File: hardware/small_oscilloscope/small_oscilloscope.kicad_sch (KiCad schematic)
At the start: 5 parts, among them J1 Conn_01x16, J2 Conn_01x16, J7 Conn_01x03, U1 CH423S

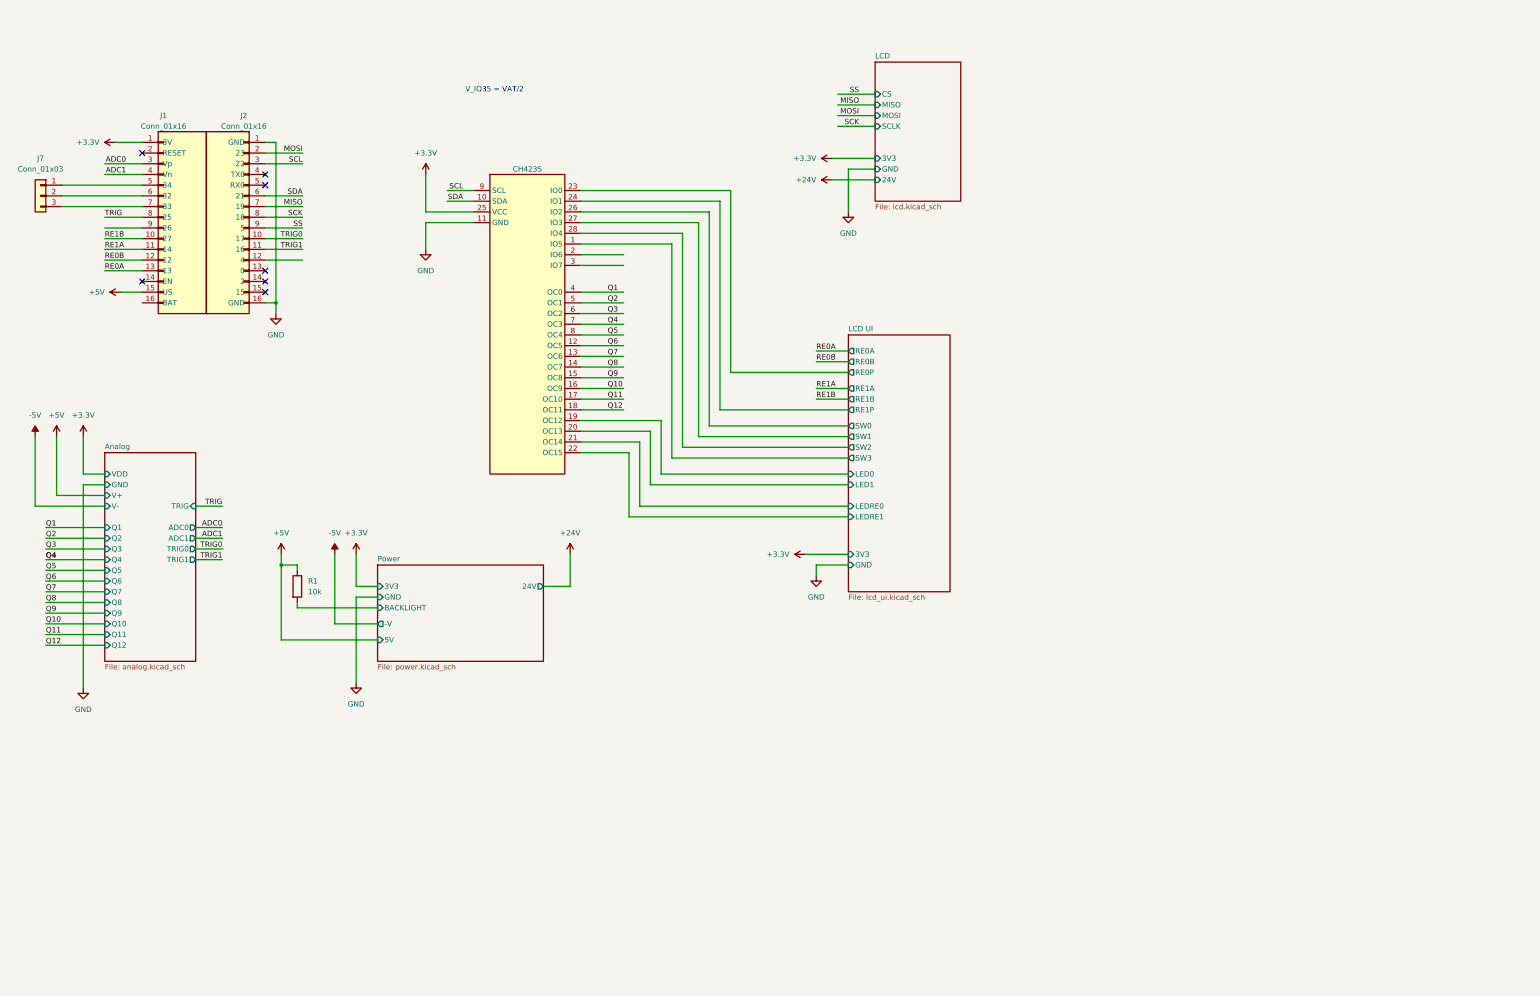
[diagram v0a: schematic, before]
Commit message: oscilliscope first success
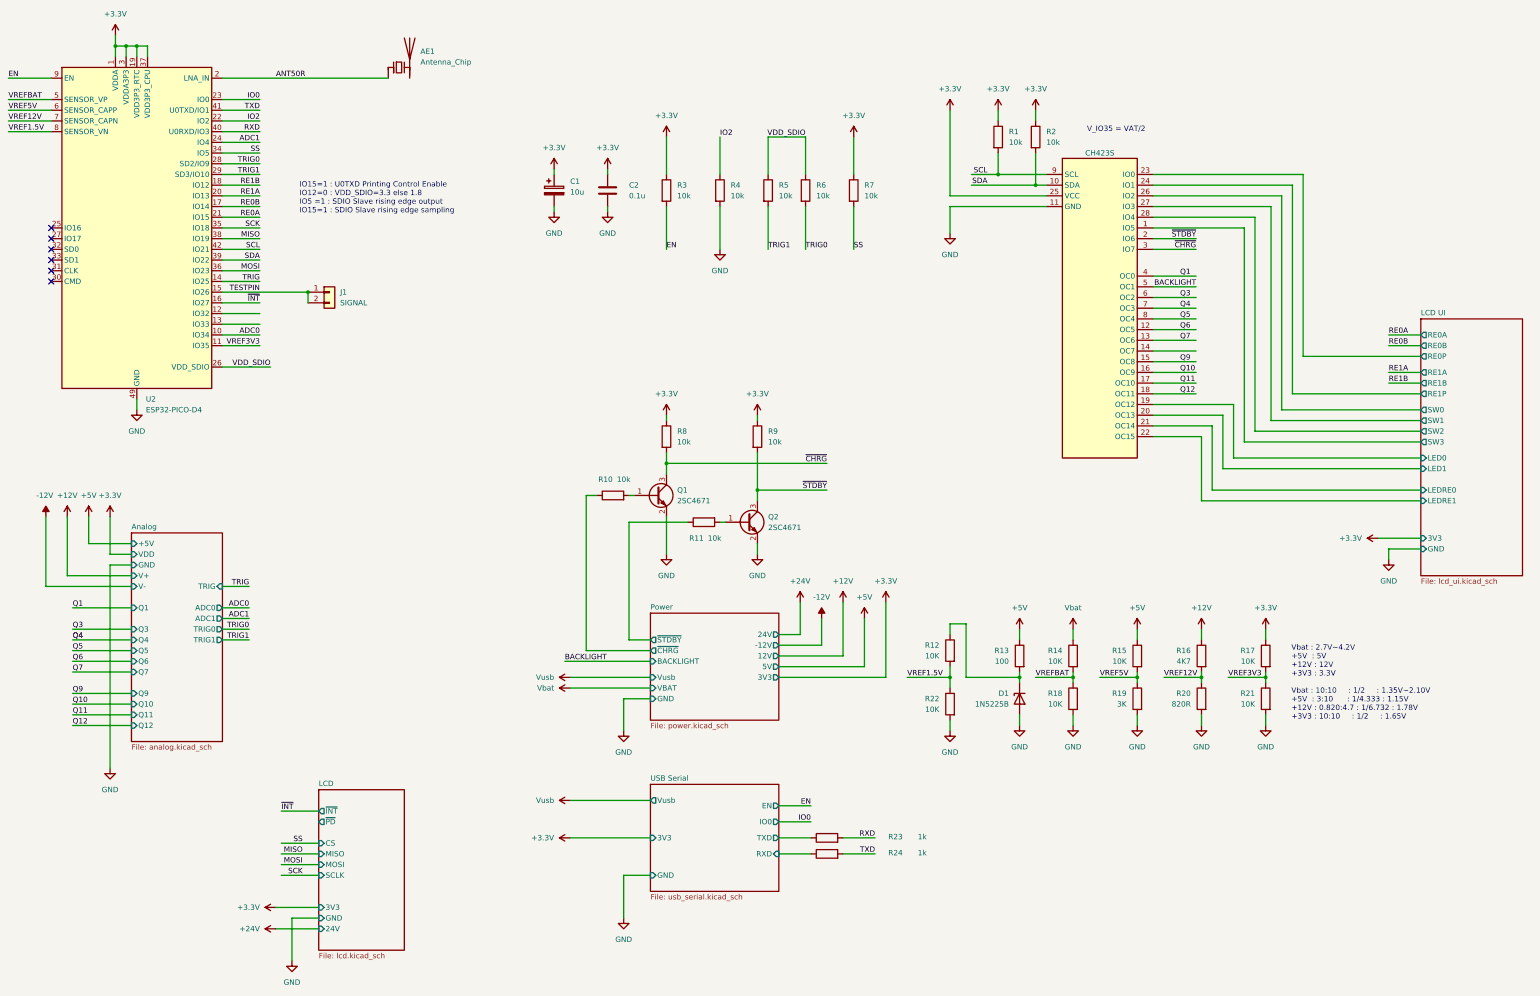
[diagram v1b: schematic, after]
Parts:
- removed J1, J2: Conn_01x16, Connector_PinSocket_2.54mm:PinSocket_1x16_P2.54mm_Vertical, symbol Connector_Generic:Conn_01x16
- removed J7: Conn_01x03, Connector_PinHeader_2.54mm:PinHeader_1x03_P2.54mm_Vertical, symbol Connector_Generic:Conn_01x03
- added AE1: Antenna_Chip, Inductor_SMD:L_1206_3216Metric_Pad1.22x1.90mm_HandSolder, symbol Device:Antenna_Chip
- added C1: 10u, Capacitor_SMD:CP_Elec_5x5.3, symbol Device:C_Polarized
- added C2: 0.1u, Capacitor_SMD:C_0402_1005Metric_Pad0.74x0.62mm_HandSolder, symbol Device:C
- added D1: 1N5225B, Diode_THT:D_A-405_P7.62mm_Horizontal, symbol Diode:1N47xxA
- added J1: SIGNAL, Connector_PinSocket_2.54mm:PinSocket_1x02_P2.54mm_Vertical, symbol Connector_Generic:Conn_01x02
- added Q1, Q2: 2SC4671, Package_TO_SOT_SMD:SOT-523, symbol Transistor_BJT:2SC4213
- added R10, R11, R2, R3, R4, R5, R6, R7, R8, R9: 10k, Resistor_SMD:R_0402_1005Metric_Pad0.72x0.64mm_HandSolder, symbol Device:R
- added R12, R14, R15, R17, R18, R21, R22: 10K, Resistor_SMD:R_0402_1005Metric_Pad0.72x0.64mm_HandSolder, symbol Device:R
- added R13: 100, Resistor_SMD:R_0603_1608Metric_Pad0.98x0.95mm_HandSolder, symbol Device:R
- added R16: 4K7, Resistor_SMD:R_0402_1005Metric_Pad0.72x0.64mm_HandSolder, symbol Device:R
- added R19: 3K, Resistor_SMD:R_0402_1005Metric_Pad0.72x0.64mm_HandSolder, symbol Device:R
- added R20: 820R, Resistor_SMD:R_0402_1005Metric_Pad0.72x0.64mm_HandSolder, symbol Device:R
- added R23, R24: 1k, Resistor_SMD:R_0603_1608Metric_Pad0.98x0.95mm_HandSolder, symbol Device:R
- added U2: ESP32-PICO-D4, Package_DFN_QFN:QFN-48-1EP_7x7mm_P0.5mm_EP5.3x5.3mm, symbol MCU_Espressif:ESP32-PICO-D4
- R1: now left out of the parts list
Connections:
- net Power/BACKLIGHT is gone; now on net SCL: R1.2
- net +3.3V: now also R1.1, C1.1, C2.1, R17.1, R2.1, R3.1, R7.1, R8.1, R9.1, U2.1 (VDDA), U2.19 (VDD3P3_RTC), U2.3 (VDDA3P3), U2.37 (VDD3P3_CPU), U2.4 (VDDA3P3), U2.43 (VDDA), U2.46 (VDDA)
- net +5V: now also R13.1, R15.1; no longer R1.1
- net ADC0: now also U2.10 (IO34)
- net ADC1: now also U2.24 (IO4)
- net GND: now also C1.2, C2.2, D1.2 (A), Q1.2 (E), Q2.2 (E), R18.2, R19.2, R20.2, R21.2, R22.2, R4.2, U2.49 (GND)
- net MISO: now also U2.38 (IO19)
- net MOSI: now also U2.36 (IO23)
- net RE0A: now also U2.21 (IO15)
- net RE0B: now also U2.17 (IO14)
- net RE1A: now also U2.20 (IO13)
- net RE1B: now also U2.18 (IO12)
- net SCK: now also U2.35 (IO18)
- net SCL: now also U2.42 (IO21)
- net SDA: now also R2.2, U2.39 (IO22)
- net SS: now also R7.2, U2.34 (IO5)
- net TRIG: now also U2.14 (IO25)
- net TRIG0: now also R6.2, U2.28 (SD2/IO9)
- net TRIG1: now also R5.2, U2.29 (SD3/IO10)
- net ~{STDBY}: now reaches U1.2 (IO6)
- net ~{STDBY}: now also Q2.3 (C), R9.2
- net ~{CHRG}: now reaches U1.3 (IO7)
- net ~{CHRG}: now also Q1.3 (C), R8.2
- net Q2 renamed BACKLIGHT
- net Q8: no longer names the net of U1.14 (OC7)
- new net: Q1.1 (B), R10.2
- new net: D1.1 (K), R12.1, R13.2
- new net: Q2.1 (B), R11.2
- new net +12V: R16.1
- new net ANT50R: AE1.1 (FEED), U2.2 (LNA_IN)
- new net EN: R3.2, U2.9 (EN)
- new net IO0: U2.23 (IO0)
- new net IO2: R4.1, U2.22 (IO2)
- new net Power/~{CHRG}: R10.1
- new net Power/~{STDBY}: R11.1
- new net RXD: R23.2, U2.40 (U0RXD/IO3)
- new net TESTPIN: J1.1 (Pin_1), J1.2 (Pin_2), U2.15 (IO26)
- new net TXD: R24.2, U2.41 (U0TXD/IO1)
- new net USB Serial/RXD: R24.1
- new net USB Serial/TXD: R23.1
- new net VDD_SDIO: R5.1, R6.1, U2.26 (VDD_SDIO)
- new net VREF1.5V: R12.2, R22.1, U2.8 (SENSOR_VN)
- new net VREF12V: R16.2, R20.1, U2.7 (SENSOR_CAPN)
- new net VREF3V3: R17.2, R21.1, U2.11 (IO35)
- new net VREF5V: R15.2, R19.1, U2.6 (SENSOR_CAPP)
- new net VREFBAT: R14.2, R18.1, U2.5 (SENSOR_VP)
- new net Vbat: R14.1
- new net ~{INT}: U2.16 (IO27)
- no-connect marks 7 -> 6
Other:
- added sheet USB Serial (usb_serial.kicad_sch)
- sheet Analog ports: added +5V; removed Q2, Q8
- sheet LCD ports: added ~{INT}, ~{PD}; removed none
- sheet Power ports: added -12V, 12V, VBAT, Vusb, ~{CHRG}, ~{STDBY}; removed -V
- note added: "IO15=1 : U0TXD Printing Control Enable IO12=0 : VDD_SDIO=3.3 else 1.8 IO5 =1 : SDIO Slave rising edge output IO15=1 : SDIO Slave rising edge sampling"
- note added: "Vbat : 2.7V~4.2V +5V : 5V +12V : 12V +3V3 : 3.3V Vbat : 10:10 : 1/2 : 1.35V~2.10V +5V : 3:10 : 1/4.333 : 1.15V +12V : 0.820:4.7 : 1/6.732 : 1.78V +3V3 : 10:10 : 1/2 : 1.65V"
